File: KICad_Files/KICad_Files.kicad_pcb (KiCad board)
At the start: 2 copper layers, 30 x 34 mm, 42 parts, among them J1 Conn_01x03_MountingPin, J2 Conn_01x03_MountingPin, J3 Conn_01x03_MountingPin, J4 USB_C_Receptacle_USB2.0_14P, J5 Conn_01x06, J6 Conn_01x06, J7 Conn_01x03_Pin, J8 Conn_01x03_Pin, SW1 RESET, SW2 RESET, U1 TPP361061-T6TR, U2 USBLC6-2SC6, U3 ESP32-C3

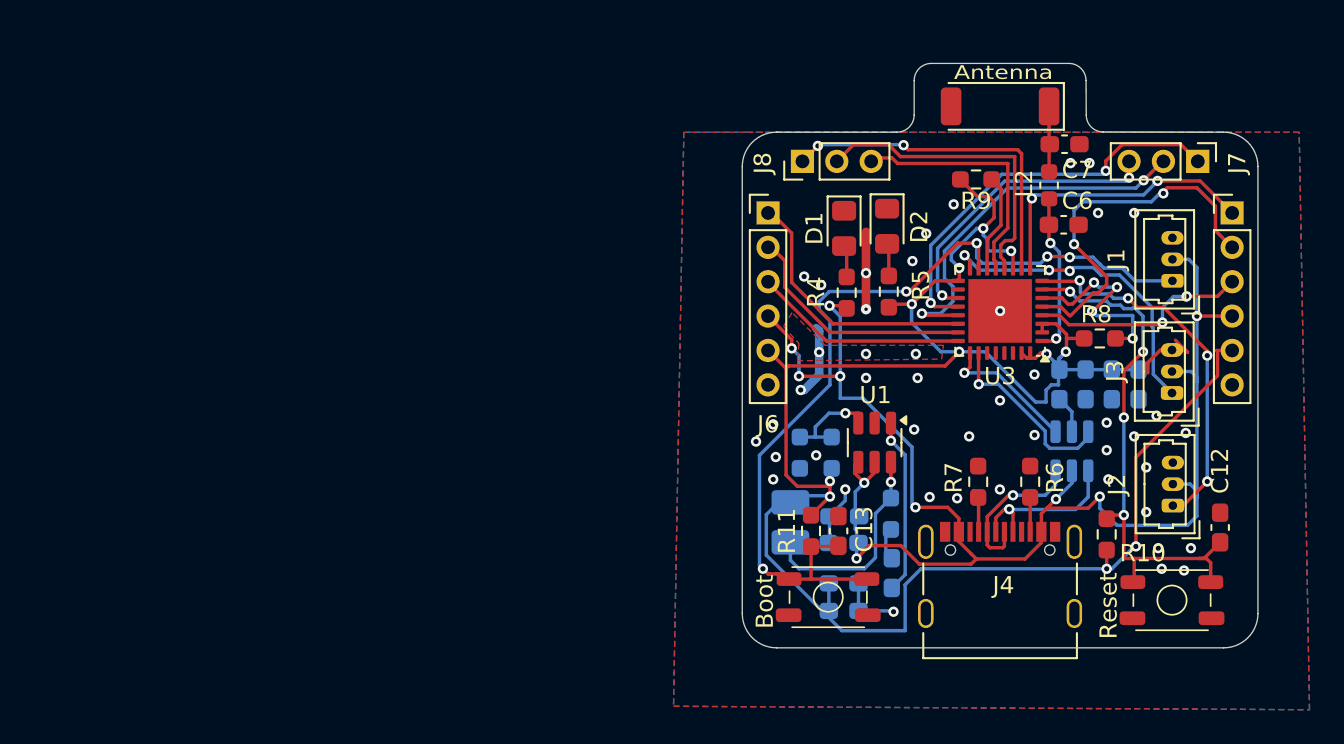
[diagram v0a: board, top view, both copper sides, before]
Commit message: rework of the PCB Layout
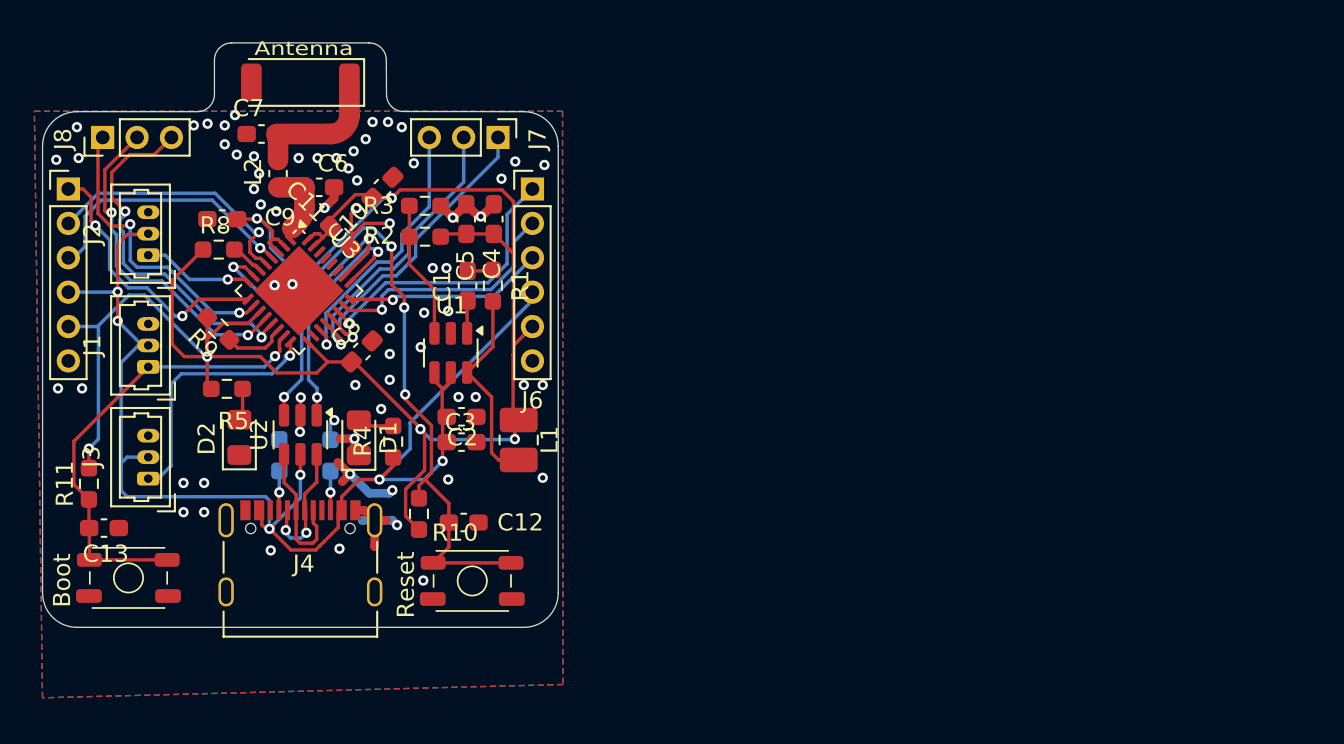
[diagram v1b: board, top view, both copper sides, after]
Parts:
- C1, C10, C11, C2, C3, C4, C5, C8, C9, L1, R1, R2, R3, U2: moved to F.Cu
- R6, R7: moved to B.Cu
- R8, R9: value 100 -> 10kΩ
- SW1: value RESET -> Reset
- SW2: value RESET -> Boot
- moved J5 67.7 mm to (93.3, 88.9)
- moved J2 61.4 mm to (98.0, 92.8)
- moved J1 59.8 mm to (98.0, 99.3)
- moved J3 59.8 mm to (98.0, 105.8)
- moved C9 52.6 mm to (102.3, 90.7), turned to 180 degrees
- moved R8 51.5 mm to (102.1, 92.4)
- moved C11 47.2 mm to (109.2, 91.7), turned to -45 degrees
- moved C7 46.7 mm to (104.5, 85.7), turned to 180 degrees
- moved R9 44.9 mm to (102.0, 97.0), turned to -45 degrees
- moved U2 44.9 mm to (106.8, 103.2)
- moved L2 44.9 mm to (105.5, 88.0)
- moved C12 44.0 mm to (116.3, 108.3), turned to 0 degrees
- moved C6 43.4 mm to (107.9, 88.8)
- moved C13 42.7 mm to (95.4, 108.6), turned to 0 degrees
- moved C10 42.5 mm to (111.6, 88.8), turned to 45 degrees
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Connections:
- J7 pad 1: /GPIO 13 -> /GPIO 14
- J7 pad 2: /GPIO 14 -> /GPIO 13
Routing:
- net /LED3: track 52.7 -> 27.0 mm, vias 5 -> 1
- net /LED2: track 22.4 -> 6.46 mm, vias 4 -> 1
- net Net-(U3-GPIO2): track 12.0 -> 1.99 mm, vias 4 -> 0
- net Net-(U3-CHIP_EN): track 31.9 -> 40.3 mm
- net Net-(U1-VBST): track 10.3 -> 1.92 mm, vias 1 -> 0
- net GND: track 22.6 -> 30.6 mm, vias 45 -> 67
- net +5V: track 85.0 -> 77.5 mm, vias 10 -> 6
- net D-: track 8.04 -> 14.6 mm, vias 1 -> 2
- net /GPIO 7: track 14.6 -> 21.1 mm, vias 0 -> 2
- net /GPIO 1: track 21.9 -> 15.5 mm, vias 2 -> 1
- net /GPIO 13: track 23.7 -> 17.4 mm, vias 2 -> 1
- net /Antenna: track 9.38 -> 4.16 mm, vias 2 -> 0
- net D+: track 10.8 -> 15.3 mm, vias 1 -> 2
- net /LED1: track 18.8 -> 15.0 mm, vias 3 -> 1
- net /GPIO 14: track 22.3 -> 18.5 mm, vias 2 -> 1
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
